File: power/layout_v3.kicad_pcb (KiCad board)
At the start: 2 copper layers, 10 parts

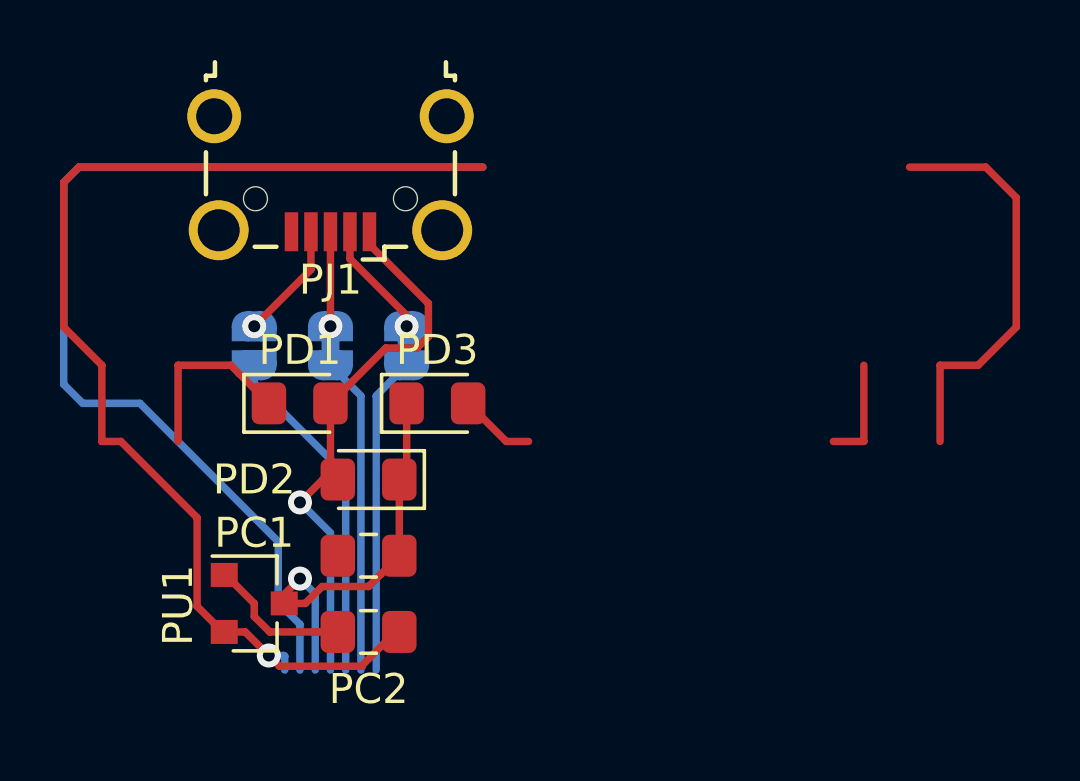
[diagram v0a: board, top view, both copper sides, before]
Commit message: Changes after combining
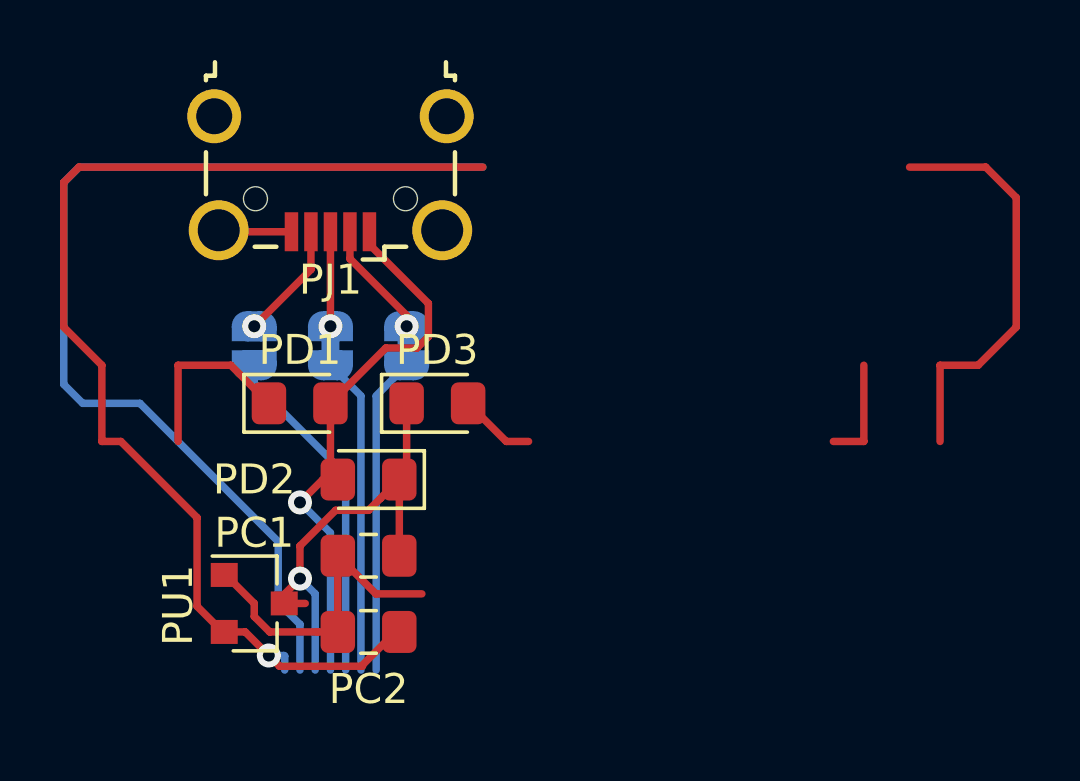
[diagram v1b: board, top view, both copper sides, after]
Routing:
- net GND: track 4.83 -> 13.1 mm
- net VREG_IN: track 14.0 -> 15.5 mm
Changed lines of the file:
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@@
     (thickness 1.6)
     (drawings 208)
-    (tracks 89)
+    (tracks 95)
     (zones 0)
     (modules 10)
@@
   (segment (start 142.24 69.335002) (end 142.754998 69.85) (width 0.25) (layer F.Cu) (net 1))
   (segment (start 141.24 67.95) (end 141.29 67.95) (width 0.25) (layer F.Cu) (net 1))
+  (segment (start 141.105 56.51) (end 141.055 56.46) (width 0.25) (layer F.Cu) (net 1))
+  (segment (start 143.48 56.51) (end 141.105 56.51) (width 0.25) (layer F.Cu) (net 1))
+  (segment (start 145.025 69.85) (end 145.025 67.31) (width 0.25) (layer F.Cu) (net 1))
+  (segment (start 145.025 67.31) (end 146.295 68.58) (width 0.25) (layer F.Cu) (net 1))
+  (segment (start 146.295 68.58) (end 147.828 68.58) (width 0.25) (layer F.Cu) (net 1))
   (segment (start 147.32 64.525) (end 147.075 64.77) (width 0.25) (layer F.Cu) (net 2))
   (segment (start 147.32 62.23) (end 147.32 64.525) (width 0.25) (layer F.Cu) (net 2))
   (segment (start 147.075 64.77) (end 147.075 67.31) (width 0.25) (layer F.Cu) (net 2))
-  (segment (start 146.451628 67.933372) (end 147.075 67.31) (width 0.25) (layer F.Cu) (net 2))
-  (segment (start 146.04999 68.33501) (end 146.451628 67.933372) (width 0.25) (layer F.Cu) (net 2))
-  (segment (start 144.50499 68.33501) (end 146.04999 68.33501) (width 0.25) (layer F.Cu) (net 2))
-  (segment (start 143.94 68.9) (end 144.50499 68.33501) (width 0.25) (layer F.Cu) (net 2))
   (segment (start 143.24 68.9) (end 143.94 68.9) (width 0.25) (layer F.Cu) (net 2))
   (via (at 143.764 68.072) (size 0.8) (drill 0.4) (layers F.Cu B.Cu) (net 2))
@@
   (segment (start 143.764 68.072) (end 144.272 68.58) (width 0.25) (layer B.Cu) (net 2))
   (segment (start 144.272 68.58) (end 144.272 71.12) (width 0.25) (layer B.Cu) (net 2))
+  (segment (start 146.04999 65.79501) (end 146.451628 65.393372) (width 0.25) (layer F.Cu) (net 2))
+  (segment (start 144.9518 65.79501) (end 146.04999 65.79501) (width 0.25) (layer F.Cu) (net 2))
+  (segment (start 146.451628 65.393372) (end 147.075 64.77) (width 0.25) (layer F.Cu) (net 2))
+  (segment (start 143.764 66.98281) (end 144.9518 65.79501) (width 0.25) (layer F.Cu) (net 2))
+  (segment (start 143.764 68.072) (end 143.764 66.98281) (width 0.25) (layer F.Cu) (net 2))
   (segment (start 147.075 69.723) (end 145.805 70.993) (width 0.25) (layer F.Cu) (net 3))
   (segment (start 167.64 59.69) (end 166.37 60.96) (width 0.25) (layer F.Cu) (net 3))
